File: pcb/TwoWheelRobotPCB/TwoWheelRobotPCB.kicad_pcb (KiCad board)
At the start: 2 copper layers, 8 parts, among them J1 Motor1, J2 Motor2, J3 L298n_sense_connector, J4 ACS712_connector, U2 L298HN, U3 ACS712_M1, U4 TXB0104D, U5 ACS712_M2

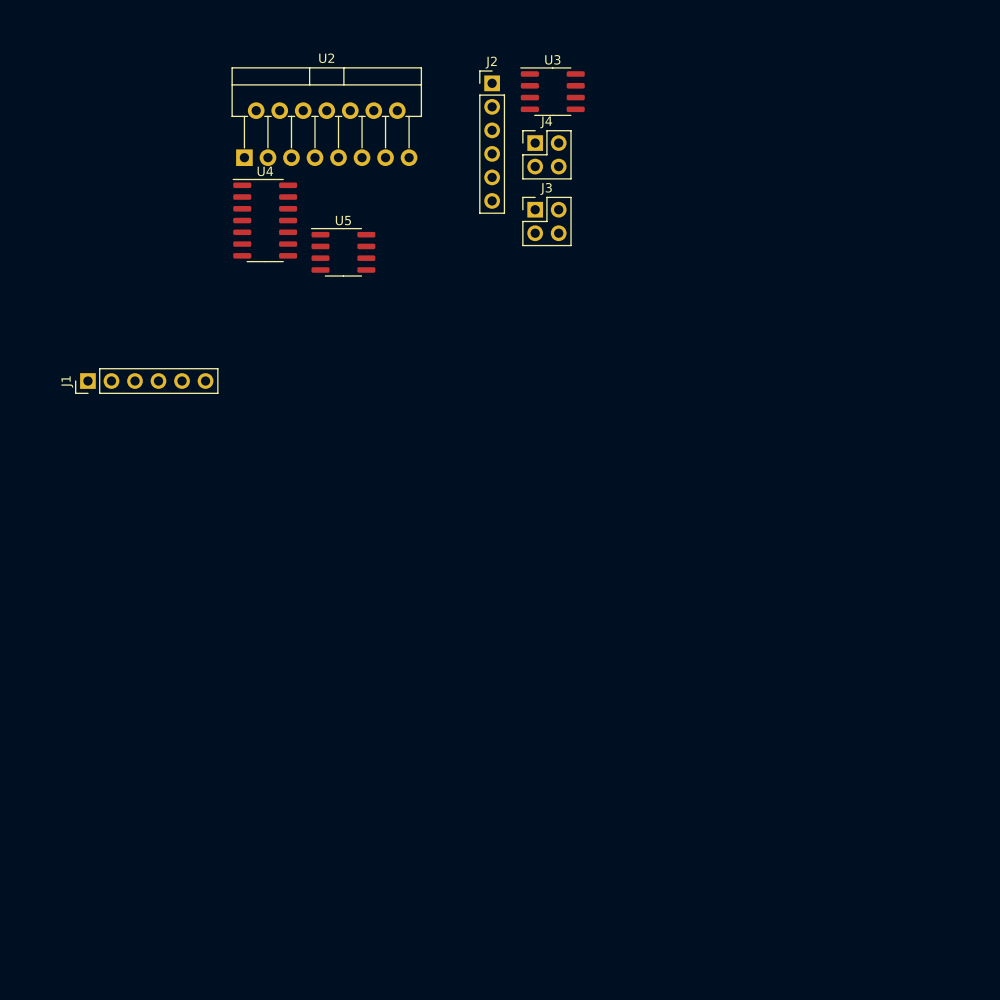
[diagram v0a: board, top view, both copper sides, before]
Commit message: pcb update
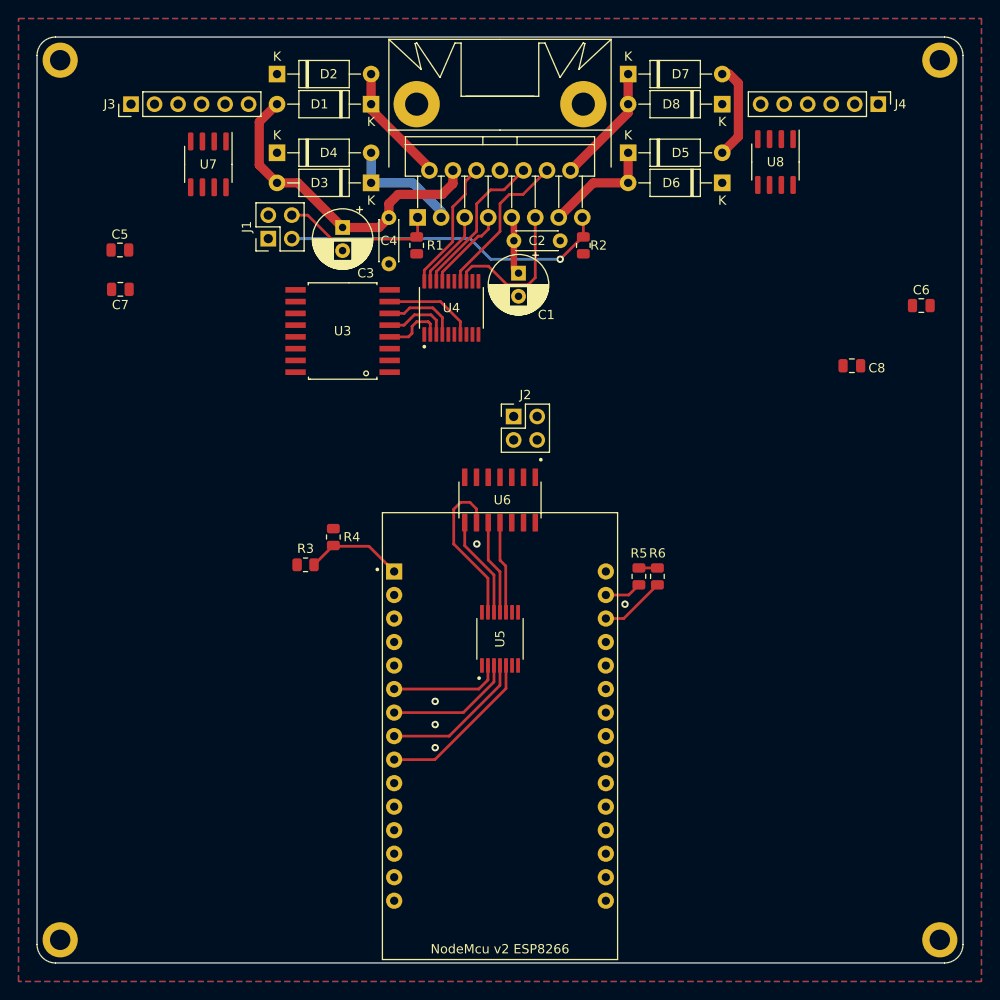
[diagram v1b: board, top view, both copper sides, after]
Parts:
- added C1: 100uF, Capacitor_THT:CP_Radial_D6.3mm_P2.50mm, F.Cu at (132.0, 85.5)
- added C2: 0.1uF, Capacitor_THT:C_Disc_D4.3mm_W1.9mm_P5.00mm, F.Cu at (131.5, 82.0)
- added C3: 100uF, Capacitor_THT:CP_Radial_D6.3mm_P2.50mm, F.Cu at (113.0, 80.6)
- added C4: 0.1uF, Capacitor_THT:C_Disc_D4.3mm_W1.9mm_P5.00mm, F.Cu at (118.0, 84.5)
- added C5: 0.1uF, Capacitor_SMD:C_0805_2012Metric, F.Cu at (89.0, 83.0)
- added C6: 0.1uF, Capacitor_SMD:C_0805_2012Metric, F.Cu at (175.5, 89.0)
- added C7: 1nF, Capacitor_SMD:C_0805_2012Metric, F.Cu at (89.0, 87.2)
- added C8: 1nF, Capacitor_SMD:C_0805_2012Metric, F.Cu at (168.0, 95.5)
- added D1: DIODE, Diode_THT:D_A-405_P10.16mm_Horizontal, F.Cu at (116.1, 67.2)
- added D2: DIODE, Diode_THT:D_A-405_P10.16mm_Horizontal, F.Cu at (105.9, 64.0)
- added D3: DIODE, Diode_THT:D_A-405_P10.16mm_Horizontal, F.Cu at (116.1, 75.8)
- added D4: DIODE, Diode_THT:D_A-405_P10.16mm_Horizontal, F.Cu at (105.9, 72.5)
- added D5: DIODE, Diode_THT:D_A-405_P10.16mm_Horizontal, F.Cu at (143.8, 72.5)
- added D6: DIODE, Diode_THT:D_A-405_P10.16mm_Horizontal, F.Cu at (154.0, 75.8)
- added D7: DIODE, Diode_THT:D_A-405_P10.16mm_Horizontal, F.Cu at (143.8, 64.0)
- added D8: DIODE, Diode_THT:D_A-405_P10.16mm_Horizontal, F.Cu at (154.0, 67.2)
- added R1: Rsa, Resistor_SMD:R_0805_2012Metric, F.Cu at (121.0, 82.5)
- added R2: Rsb, Resistor_SMD:R_0805_2012Metric, F.Cu at (139.0, 82.5)
- added R3: 10k, Resistor_SMD:R_0805_2012Metric, F.Cu at (109.0, 117.0)
- added R4: 18k, Resistor_SMD:R_0805_2012Metric, F.Cu at (112.0, 114.0)
- added R5: 2k2, Resistor_SMD:R_0805_2012Metric, F.Cu at (145.0, 118.2)
- added R6: 2k2, Resistor_SMD:R_0805_2012Metric, F.Cu at (147.0, 118.2)
- added REF**: MountingHole_2.2mm_M2_DIN965_Pad, MountingHole:MountingHole_2.2mm_M2_DIN965_Pad, F.Cu at (177.5, 157.5)
- added REF**: MountingHole_2.2mm_M2_DIN965_Pad, MountingHole:MountingHole_2.2mm_M2_DIN965_Pad, F.Cu at (82.5, 157.5)
- added REF**: MountingHole_2.2mm_M2_DIN965_Pad, MountingHole:MountingHole_2.2mm_M2_DIN965_Pad, F.Cu at (82.5, 62.5)
- added REF**: Heatsink_Fischer_SK104-STC-STIC_35x13mm_2xDrill2.5mm, Heatsink:Heatsink_Fischer_SK104-STC-STIC_35x13mm_2xDrill2.5mm, F.Cu at (130.0, 67.2)
- added REF**: MountingHole_2.2mm_M2_DIN965_Pad, MountingHole:MountingHole_2.2mm_M2_DIN965_Pad, F.Cu at (177.5, 62.5)
- added U1: NodeMCU1.0(ESP-12E), NodemcuESP8266_footprint:MODULE_ZC563900, F.Cu at (130.0, 135.5)
- added U6: MCP3004, MCP3004_footprint:SOIC127P600X175-14N, F.Cu at (130.0, 110.0)
- added U7: ACS712_M1, Package_SO:SOIC-8_3.9x4.9mm_P1.27mm, F.Cu at (98.5, 73.8)
- added U8: ACS712_M2, Package_SO:SOIC-8_3.9x4.9mm_P1.27mm, F.Cu at (159.8, 73.5)
- J1: value Motor1 -> L298n_sense_connector; footprint Connector_PinHeader_2.54mm:PinHeader_1x06_P2.54mm_Vertical -> Connector_PinHeader_2.54mm:PinHeader_2x02_P2.54mm_Vertical
- J2: value Motor2 -> ACS712_connector; footprint Connector_PinHeader_2.54mm:PinHeader_1x06_P2.54mm_Vertical -> Connector_PinHeader_2.54mm:PinHeader_2x02_P2.54mm_Vertical
- J3: value L298n_sense_connector -> Motor1; footprint Connector_PinHeader_2.54mm:PinHeader_2x02_P2.54mm_Vertical -> Connector_PinHeader_2.54mm:PinHeader_1x06_P2.54mm_Vertical
- J4: value ACS712_connector -> Motor2; footprint Connector_PinHeader_2.54mm:PinHeader_2x02_P2.54mm_Vertical -> Connector_PinHeader_2.54mm:PinHeader_1x06_P2.54mm_Vertical
- U3: value ACS712_M1 -> PCF8574; footprint Package_SO:SOIC-8_3.9x4.9mm_P1.27mm -> PCF8574:SO16W
- U4: value TXB0104D -> TXB0108DQSR; footprint Package_SO:SOIC-14_3.9x8.7mm_P1.27mm -> TXB0108_TSOP20_fotprint:SOP65P640X120-20N
- U5: value ACS712_M2 -> TXB0104D; footprint Package_SO:SOIC-8_3.9x4.9mm_P1.27mm -> TXB0104_TSOP14_footprint:SOP65P640X120-14N
- moved J3 45.1 mm to (90.2, 67.2), turned to 90 degrees
- moved U5 45.0 mm to (130.0, 125.0), turned to 90 degrees
- moved J4 37.3 mm to (170.8, 67.2), turned to -90 degrees
- moved J2 36.1 mm to (131.5, 101.0)
- moved U3 34.4 mm to (113.0, 91.8), turned to 90 degrees
- moved J1 24.8 mm to (105.0, 81.8)
- moved U4 22.2 mm to (124.8, 89.2), turned to 90 degrees
- moved U2 19.8 mm to (121.1, 79.5)
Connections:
- J1 pad 1: unconnected-(J1-Pad1) -> ADC1
- J1 pad 2: unconnected-(J1-Pad2) -> ADC2
- J1 pad 3: unconnected-(J1-Pad3) -> Sense_B
- J1 pad 4: unconnected-(J1-Pad4) -> Sense_A
- J2 pad 1: unconnected-(J2-Pad1) -> ADC1
- J2 pad 2: unconnected-(J2-Pad2) -> ADC2
- J2 pad 3: unconnected-(J2-Pad3) -> VIOUT_M2
- J2 pad 4: unconnected-(J2-Pad4) -> VIOUT_M1
- J3 pad 1: ADC1 -> M1-
- J3 pad 2: ADC2 -> GND
- J3 pad 3: Sense_B -> M1_C1
- J3 pad 4: Sense_A -> M1_C2
- J4 pad 1: ADC1 -> M2-
- J4 pad 2: ADC2 -> GND
- J4 pad 3: VIOUT_M2 -> M2_C1
- J4 pad 4: VIOUT_M1 -> M2_C2
- U2 pad 13: OUT3 -> OUT2
- U2 pad 14: OUT4 -> M2-
- U2 pad 3: OUT2 -> M1-
- U2 pad 9: +3V3 -> +5V
- U3 pad 1: Net-(U3-Pad1) -> GND
- U3 pad 2: Net-(U3-Pad1) -> GND
- U3 pad 3: Net-(U3-Pad3) -> GND
- U3 pad 4: Net-(U3-Pad3) -> dir1_M1
- U3 pad 5: GND -> dir1_M2
- U3 pad 6: Net-(U3-Pad6) -> dir2_M1
- U3 pad 7: VIOUT_M1 -> dir2_M2
- U3 pad 8: +5V -> GND
- U4 pad 1: +3V3 -> pwm1
- U4 pad 10: CS -> unconnected-(U4-Pad10)
- U4 pad 11: Din -> unconnected-(U4-Pad11)
- U4 pad 12: Dout -> unconnected-(U4-Pad12)
- U4 pad 13: CLK -> PWM2
- U4 pad 14: +5V -> DIR2_M2
- U4 pad 2: SCLK -> dir1_M1
- U4 pad 3: MISO -> dir1_M2
- U4 pad 4: MOSI -> dir2_M1
- U4 pad 5: CS_ -> +3V3
- U4 pad 6: unconnected-(U4-Pad6) -> +3V3
- U4 pad 7: GND -> dir2_M2
- U4 pad 8: +3V3 -> pwm2
- U5 pad 1: Net-(U5-Pad1) -> +3V3
- U5 pad 2: Net-(U5-Pad1) -> MOSI
- U5 pad 3: Net-(U5-Pad3) -> CS_
- U5 pad 4: Net-(U5-Pad3) -> MISO
- U5 pad 5: GND -> SCLK
- U5 pad 6: Net-(C8-Pad1) -> unconnected-(U5-Pad6)
- U5 pad 7: VIOUT_M2 -> GND
- U5 pad 8: +5V -> +3V3
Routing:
- net VS: track 0.00 -> 45.7 mm
- net Sense_B: track 0.00 -> 35.6 mm, vias 0 -> 1
- net SCLK: track 0.00 -> 17.7 mm
- net Din: track 0.00 -> 17.2 mm
- net Sense_A: track 0.00 -> 16.8 mm
- net DIR1_M2: track 0.00 -> 16.7 mm
- net DIR2_M2: track 0.00 -> 16.7 mm
- net PWM2: track 0.00 -> 16.4 mm
- net MISO: track 0.00 -> 15.8 mm
- net PWM1: track 0.00 -> 14.3 mm
- net CS_: track 0.00 -> 13.9 mm
- net OUT1: track 0.00 -> 13.0 mm
- net M2-: track 0.00 -> 13.0 mm
- net M1-: track 0.00 -> 12.7 mm
- net OUT2: track 0.00 -> 12.3 mm
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- added copper zone on B.Cu, net GND
- added copper zone on F.Cu, net GND
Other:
- board outline added: 100 x 100 mm
- board text added: "NodeMcu v2 ESP8266"
